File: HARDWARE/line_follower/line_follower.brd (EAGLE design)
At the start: 68.6 x 88.9 mm, 70 parts, among them IC1 L3GD20HSMD, IC2 L6205, IC3 ATMEGA328PMA, IC4 LF33, J1 FFC2B05-10-X_REVC, J2 FFC2B05-10-X_REVC, Q1 10MHz, T1 ELPT15-21C, T2 ELPT15-21C, T3 ELPT15-21C, T4 ELPT15-21C, T5 ELPT15-21C, T6 ELPT15-21C, X1 MINI-USB-SCHIELD-32005-201

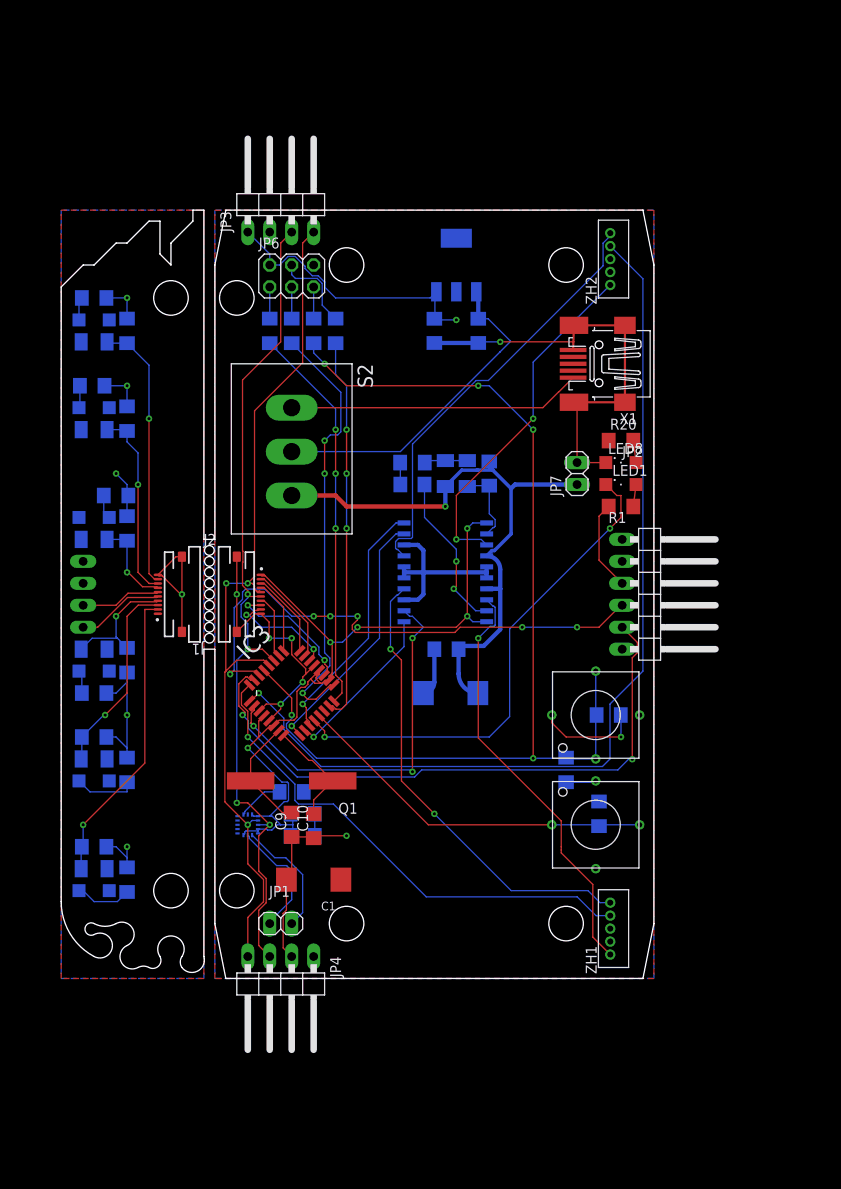
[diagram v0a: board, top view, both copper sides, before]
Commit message: common
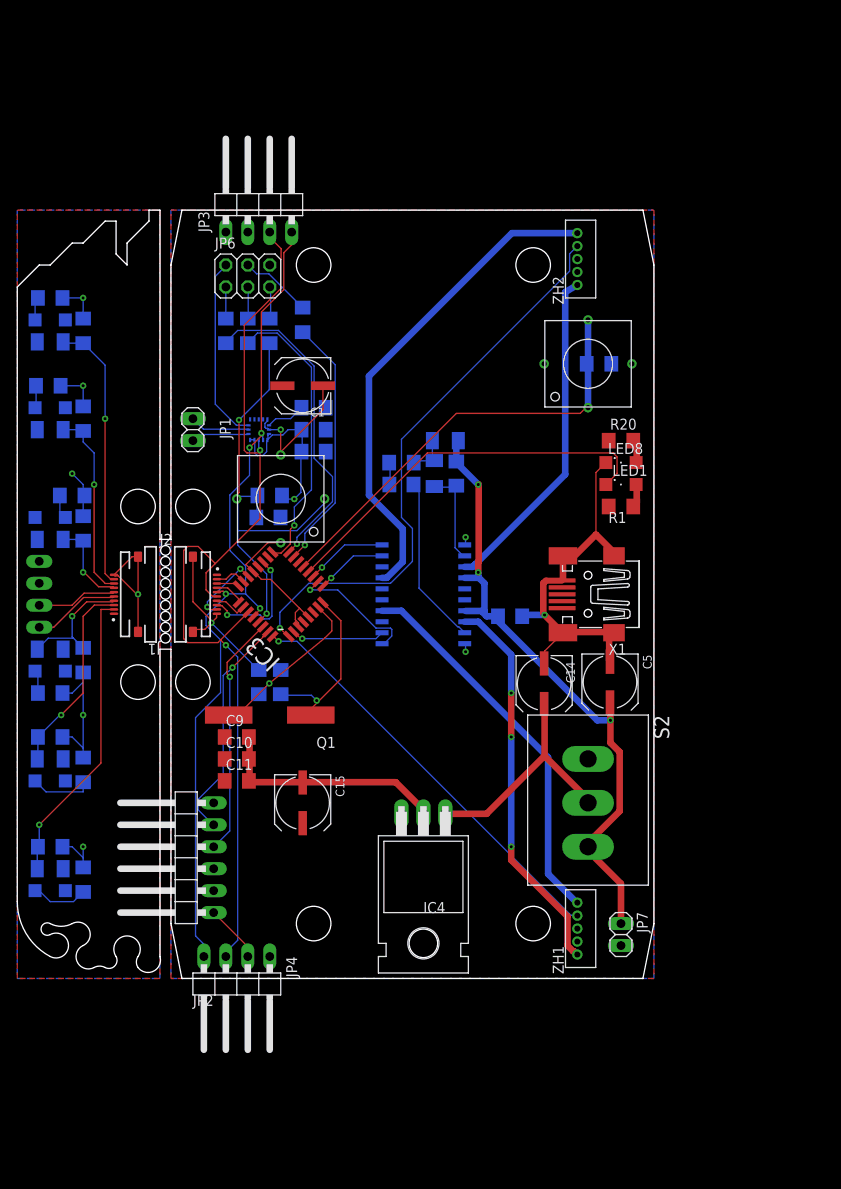
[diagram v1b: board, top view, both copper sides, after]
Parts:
- added C14, C15: 100u, rcl:UD-6,3X5,8_NICHICON
- added C16: 100n, rcl:C1206
- C1: value 10u -> 100u; device rcl:SMC_D -> rcl:UD-6,3X5,8_NICHICON
- C10, C9: value 22p -> 100n
- C12, C13: value 100n -> 22p
- C5: device rcl:SMC_D -> rcl:UD-6,3X5,8_NICHICON
- IC4: device linear:SOT223 -> linear:TO220H
- JP7: value 3S/4S -> 3S
- R10, R12, R14, R4, R6, R8: value 220 -> 120
- R20: value 220 -> 470
- X1: value MINI-USB-SCHIELD-32005-201 -> MINI-USB-SCHIELD-32005-301; device con-cypressindustries:32005-201 -> con-cypressindustries:32005-301
- moved IC4 73.8 mm to (41.9, 8.89), flipped to the top, turned to 180 degrees
- moved JP2 62.8 mm to (13.8, 14.0), turned to 90 degrees
- moved C11 59.1 mm to (20.3, 22.9), flipped to the top, turned to 0 degrees
- moved JP1 58.0 mm to (15.2, 63.5), turned to 270 degrees
- moved C1 57.2 mm to (27.9, 68.6)
- moved JP7 53.6 mm to (64.8, 5.08), turned to 270 degrees
- moved S1 53.3 mm to (61.0, 71.1), turned to 90 degrees
- moved S2 53.2 mm to (61.0, 20.3)
- moved R2 52.1 mm to (62.2, 71.1), turned to 180 degrees
- moved R21 46.7 mm to (24.1, 55.9), turned to 0 degrees
- moved IC1 45.7 mm to (22.9, 63.5), turned to 90 degrees
- moved C12 45.4 mm to (22.9, 34.3)
- moved C4 44.5 mm to (29.2, 66.0)
- moved C2 44.5 mm to (29.2, 61.0)
- moved C3 44.5 mm to (29.2, 63.5)
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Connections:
- new net V+: X1.1
- net !RESET: now also C16.1; no longer C13.1
- net GND: now also C10.2, C12.1, C13.1, C14.-, C15.-, C16.2, C9.2, IC4.2; no longer C10.1, C12.2, C13.2, C9.1, IC4.4
- net N$10: now also C14.+; no longer C11.1
- net VCC: now also C10.1, C11.1, C15.+, C9.1; no longer C12.1
- net VUSB: no longer X1.1
- net XTAL1: now also C12.2; no longer C9.2
- net XTAL2: now also C13.2; no longer C10.2
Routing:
- net VCC: track 141.3 -> 44.2 mm, vias 6 -> 3
- net !RESET: track 124.1 -> 52.8 mm, vias 5 -> 2
- net TX: track 72.1 -> 26.5 mm, vias 2 -> 1
- net INT1: track 109.9 -> 66.5 mm
- net RX: track 63.9 -> 28.1 mm, vias 6 -> 1
- net VUSB: track 34.0 -> 0.00 mm
- net DIRA: track 43.7 -> 10.8 mm, vias 3 -> 1
- net OC0B: track 29.6 -> 8.30 mm
- net DIRB: track 29.2 -> 9.49 mm
- net SCK: track 50.4 -> 33.5 mm, vias 3 -> 1
- net MOSI: track 44.7 -> 29.5 mm, vias 3 -> 1
- net SDA: track 98.2 -> 113.1 mm, vias 4 -> 2
- net GND: track 148.6 -> 133.9 mm, vias 8 -> 3
- net LED: track 58.0 -> 45.3 mm, vias 2 -> 0
- net N$10: track 38.8 -> 27.8 mm
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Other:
- board size 68.6 x 88.9 mm -> 73.7 x 88.9 mm

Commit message: common
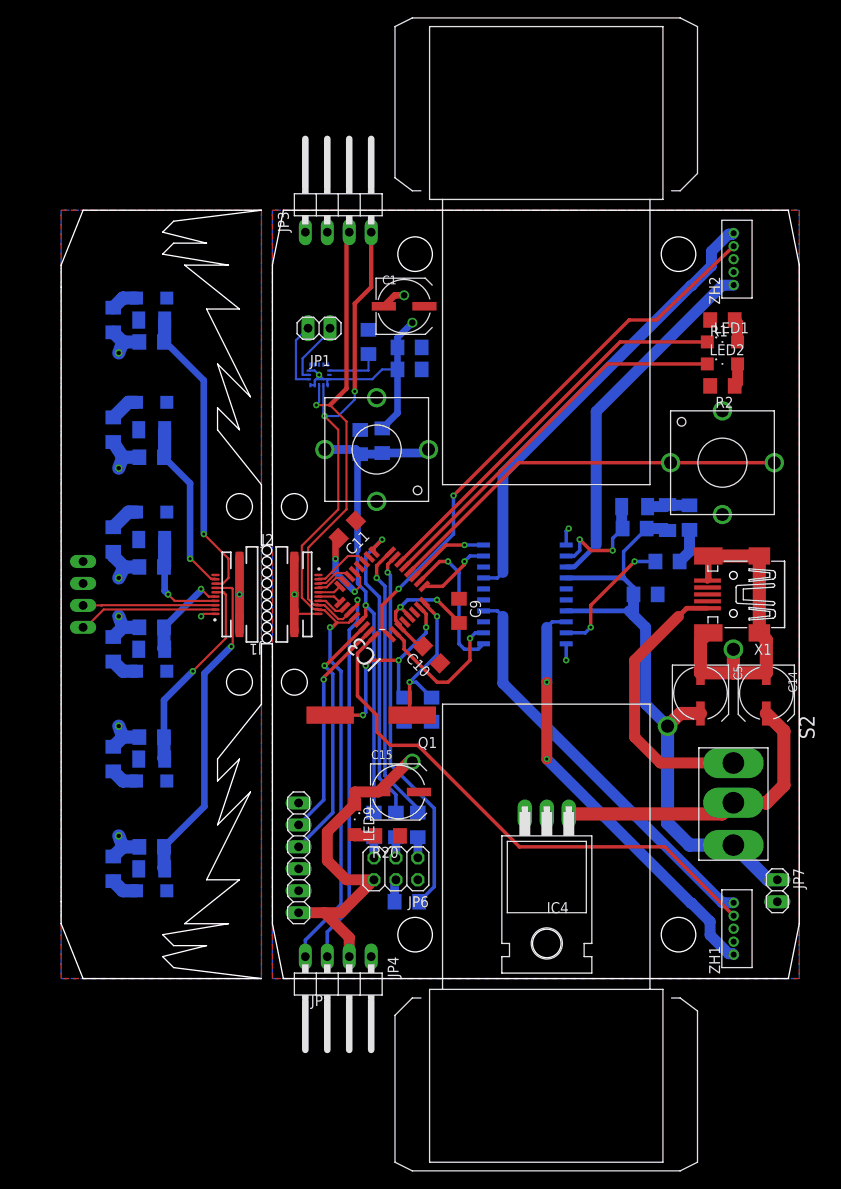
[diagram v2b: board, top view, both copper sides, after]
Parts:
- added LED9: Orange, led:SML1206
- JP2: device pinhead:1X06/90 -> pinhead:1X06
- LED2: value White -> Purple
- LED8: value Orange -> White
- R2: value 1k -> 680
- moved LED2 98.8 mm to (76.5, 71.1), flipped to the top
- moved JP6 70.7 mm to (38.7, 12.7), turned to 180 degrees
- moved R19 68.4 mm to (40.0, 8.88), turned to 180 degrees
- moved R18 61.3 mm to (41.3, 17.8), turned to 90 degrees
- moved R17 59.7 mm to (38.7, 17.8), turned to 90 degrees
- moved R16 58.4 mm to (36.2, 17.8), turned to 90 degrees
- moved LED8 57.5 mm to (10.5, 78.7), flipped to the bottom
- moved R20 53.1 mm to (37.8, 16.5), turned to 180 degrees
- moved R3 33.9 mm to (72.7, 53.3), turned to 90 degrees
- moved C8 32.1 mm to (70.2, 48.2), turned to 180 degrees
- moved C11 31.8 mm to (33.1, 52.0), turned to 225 degrees
- moved C9 29.6 mm to (46.0, 42.5), turned to 270 degrees
- moved D1 27.2 mm to (70.2, 53.3), turned to 90 degrees
- moved C14 25.7 mm to (81.6, 33.0)
- moved C10 25.6 mm to (42.9, 37.5), turned to 135 degrees
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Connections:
- removed net !SS: IC3.14
- removed net LED: IC3.12, LED1.C
- removed net V+: X1.1
- new net LEDA: IC3.13, LED2.C
- new net LEDB: IC3.14, LED1.C
- new net N$13: LED2.A, R2.1
- net ADC0: now also J2.4; no longer J2.2
- net ADC1: now also J2.5; no longer J2.3
- net ADC2: now also J2.6; no longer J2.4
- net ADC6: now also J2.2; no longer J2.8
- net ADC7: now also J2.3; no longer J2.9
- net F_ADC0: now also J1.7; no longer J1.2
- net F_ADC1: now also J1.6; no longer J1.3
- net F_ADC2: now also J1.5; no longer J1.4
- net F_ADC3: now also J1.4; no longer J1.7
- net F_ADC6: now also J1.9; no longer J1.8
- net F_ADC7: now also J1.8; no longer J1.9
- net F_GND: now also J1.1, LED8.C; no longer J1.10, LED2.C
- net F_SCL: now also J1.2; no longer J1.5
- net F_SDA: now also J1.3; no longer J1.6
- net F_VCC: now also J1.10; no longer J1.1
- net GND: now also LED9.C, S1.B@1, S1.B@2; no longer LED8.C, R2.2
- net N$1: now also LED5.A; no longer LED4.A
- net N$12: now also LED6.A; no longer LED5.A
- net N$22: now also LED8.A; no longer LED7.A
- net N$30: now also LED7.A; no longer LED6.A
- net N$36: now also LED9.A; no longer LED8.A
- net N$43: now also LED4.A; no longer LED3.A
- net N$47: now also LED3.A; no longer LED2.A
- net SCL: now also J2.9; no longer J2.5
- net SDA: now also J2.8; no longer J2.6
- net USR: now also IC3.12; no longer IC3.13, R2.1
- net VCC: now also R2.2; no longer S1.B@1, S1.B@2
- net VUSB: now also X1.1
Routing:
- net LEDB: track 0.00 -> 46.1 mm
- net LED: track 45.3 -> 0.00 mm
- net LEDA: track 0.00 -> 44.7 mm
- net VUSB: track 0.00 -> 32.5 mm
- net GND: track 133.9 -> 119.1 mm, vias 3 -> 8
- net INT0: track 48.6 -> 62.8 mm, vias 1 -> 0
- net MOSI: track 29.5 -> 43.2 mm
- net SDA: track 113.1 -> 100.6 mm
- net VCC: track 44.2 -> 32.2 mm, vias 3 -> 4
- net N$10: track 27.8 -> 35.4 mm
- net ADC6: track 14.2 -> 6.72 mm, vias 2 -> 0
- net DIRA: track 10.8 -> 17.1 mm
- net F_VCC: track 36.3 -> 30.2 mm, vias 5 -> 6
- net F_SDA: track 9.28 -> 15.3 mm
- net F_SCL: track 10.1 -> 16.2 mm
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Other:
- board size 73.7 x 88.9 mm -> 85.4 x 88.9 mm
- board text added: "/home/arch/Documents/proj/slate_vixen/HARDWARE/line_follower/printing/dragon_head.bmp"
